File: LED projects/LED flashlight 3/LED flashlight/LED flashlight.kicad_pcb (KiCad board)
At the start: 2 copper layers, 37.1 x 17.5 mm, 16 parts, among them P1 USB_C_Plug_USB2.0, SW1 SW_Push, U1 TP4056

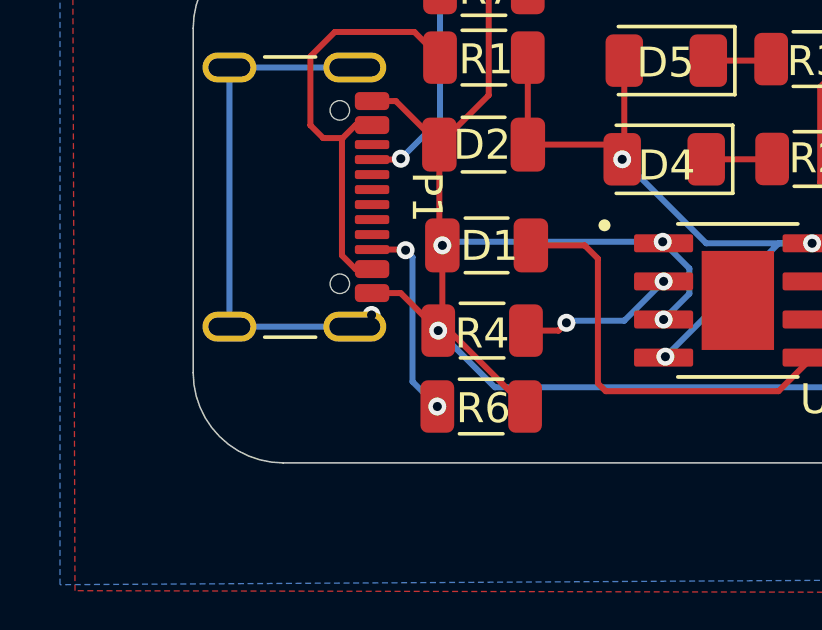
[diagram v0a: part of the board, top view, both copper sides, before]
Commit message: update
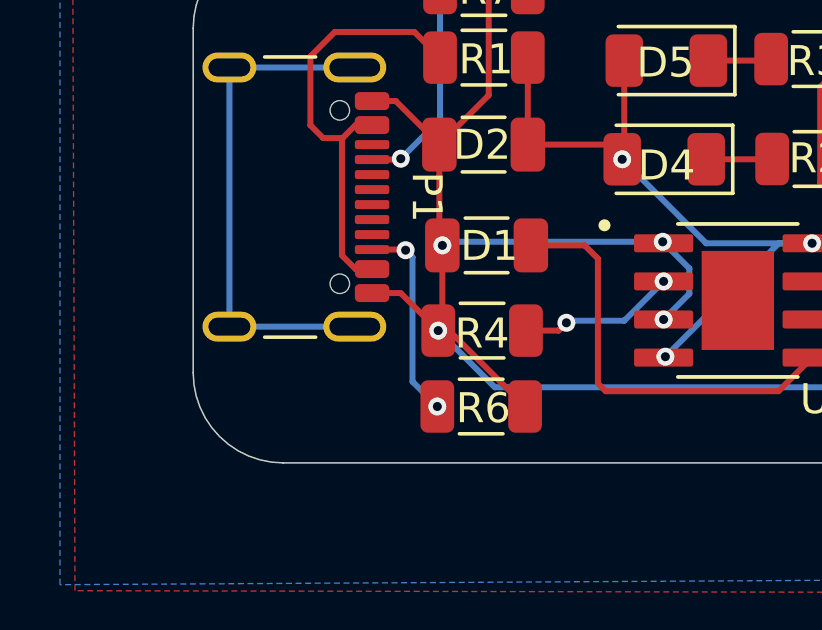
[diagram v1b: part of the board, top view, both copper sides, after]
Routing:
- net unconnected-(P1-SHIELD-PadS1): vias 1 -> 0
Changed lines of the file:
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@@
 		(net 8)
-	)
-	(via
-		(at 129.725 95.47)
-		(size 0.6)
-		(drill 0.3)
-		(layers "F.Cu" "B.Cu")
-		(net 9)
 	)
 	(segment
